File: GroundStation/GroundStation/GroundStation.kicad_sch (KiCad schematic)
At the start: 72 parts, among them J1 SD_Card_Receptacle, J101 Conn_01x02, J102 Conn_01x02, J3 Conn_01x04, J4 Conn_Coaxial, J5 Conn_01x02, P1 USB_C_Plug_USB2.0, Q1 AO3401A, SW1 SW_Push, U1 STM32F103C8Tx, U10 E22-400T30S, U101 LD1117S33TR_SOT223, U11 E80-900M23313S, U9 NEO-M9N-00B, Y1 8Mhz

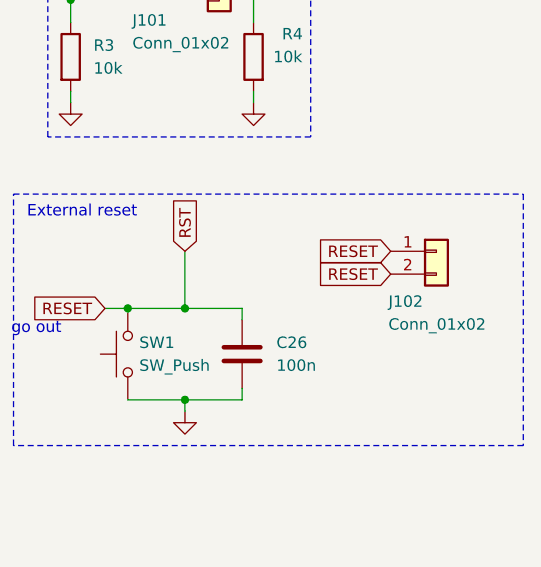
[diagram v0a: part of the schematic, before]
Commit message: Groung garber
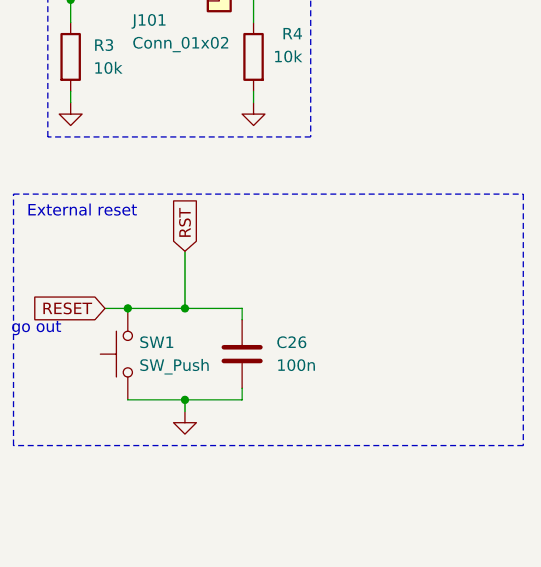
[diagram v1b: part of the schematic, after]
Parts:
- removed J102: Conn_01x02, Connector_PinHeader_2.54mm:PinHeader_1x02_P2.54mm_Vertical, symbol Connector_Generic:Conn_01x02
- C101: footprint Capacitor_SMD:C_0805_2012Metric_Pad1.18x1.45mm_HandSolder -> Capacitor_SMD:smd7343
- C22, C24: footprint Capacitor_SMD:C_0805_2012Metric_Pad1.18x1.45mm_HandSolder -> Capacitor_SMD:SMD3528
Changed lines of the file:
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@@
 		)
 	)
-	(global_label "RESET"
-		(shape input)
-		(at 417.83 302.26 180)
-		(fields_autoplaced yes)
-		(effects
-			(font
-				(size 1.27 1.27)
-			)
-			(justify right)
-		)
-		(property "Intersheetrefs" "${INTERSHEET_REFS}"
-			(at 409.0997 302.26 0)
-			(effects
-				(font
-					(size 1.27 1.27)
-				)
-				(justify right)
-				(hide yes)
-			)
-		)
-	)
 	(global_label "USART2_LoRa1_M1"
 		(shape input)
@@
 		)
 	)
-	(global_label "RESET"
-		(shape input)
-		(at 417.83 304.8 180)
-		(fields_autoplaced yes)
-		(effects
-			(font
-				(size 1.27 1.27)
-			)
-			(justify right)
-		)
-		(property "Intersheetrefs" "${INTERSHEET_REFS}"
-			(at 409.0997 304.8 0)
-			(effects
-				(font
-					(size 1.27 1.27)
-				)
-				(justify right)
-				(hide yes)
-			)
-		)
-	)
 	(global_label "USART1_GPS_RX"
 		(shape input)
@@
 	)
 	(symbol
-		(lib_id "Connector_Generic:Conn_01x02")
-		(at 422.91 302.26 0)
-		(unit 1)
-		(exclude_from_sim no)
-		(in_bom yes)
-		(on_board yes)
-		(dnp no)
-		(property "Reference" "J102"
-			(at 417.576 307.848 0)
-			(effects
-				(font
-					(size 1.27 1.27)
-				)
-				(justify left)
-			)
-		)
-		(property "Value" "Conn_01x02"
-			(at 417.576 310.388 0)
-			(effects
-				(font
-					(size 1.27 1.27)
-				)
-				(justify left)
-			)
-		)
-		(property "Footprint" "Connector_PinHeader_2.54mm:PinHeader_1x02_P2.54mm_Vertical"
-			(at 422.91 302.26 0)
-			(effects
-				(font
-					(size 1.27 1.27)
-				)
-				(hide yes)
-			)
-		)
-		(property "Datasheet" "~"
-			(at 422.91 302.26 0)
-			(effects
-				(font
-					(size 1.27 1.27)
-				)
-				(hide yes)
-			)
-		)
-		(property "Description" "Generic connector, single row, 01x02, script generated (kicad-library-utils/schlib/autogen/connector/)"
-			(at 422.91 302.26 0)
-			(effects
-				(font
-					(size 1.27 1.27)
-				)
-				(hide yes)
-			)
-		)
-		(pin "2"
-		)
-		(pin "1"
-		)
-		(instances
-			(project "GroundStation"
-				(path "/5c79a8d7-118d-4f5f-b925-c53bb7ecf529"
-					(reference "J102")
-					(unit 1)
-				)
-			)
-		)
-	)
-	(symbol
 		(lib_id "power:GND")
 		(at 133.35 54.61 0)
@@
 			)
 		)
-		(property "Footprint" "Capacitor_SMD:C_0805_2012Metric_Pad1.18x1.45mm_HandSolder"
+		(property "Footprint" "Capacitor_SMD:SMD3528"
 			(at 124.7648 300.99 0)
 			(effects
@@
 			)
 		)
-		(property "Footprint" "Capacitor_SMD:C_0805_2012Metric_Pad1.18x1.45mm_HandSolder"
+		(property "Footprint" "Capacitor_SMD:smd7343"
 			(at 61.9252 238.76 0)
 			(effects
@@
 			)
 		)
-		(property "Footprint" "Capacitor_SMD:C_0805_2012Metric_Pad1.18x1.45mm_HandSolder"
+		(property "Footprint" "Capacitor_SMD:SMD3528"
 			(at 134.9248 300.99 0)
 			(effects
